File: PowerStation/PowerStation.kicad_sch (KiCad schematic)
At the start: 0 parts

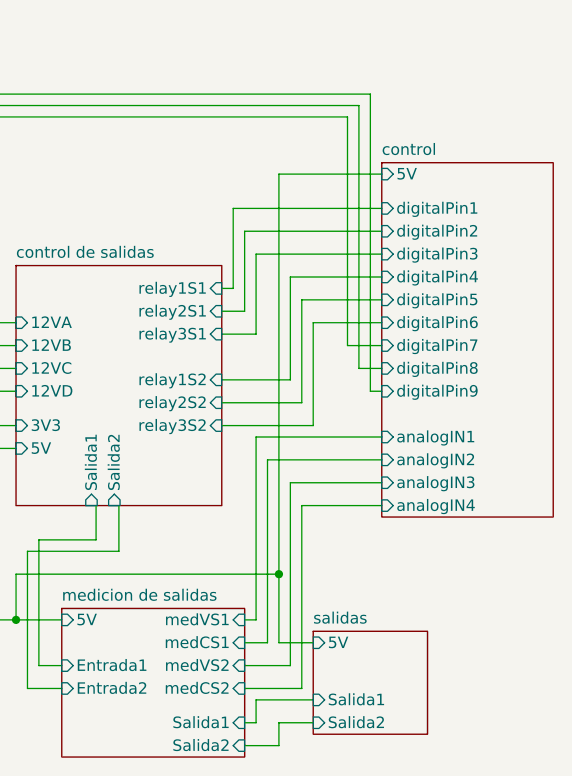
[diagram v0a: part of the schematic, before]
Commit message: correccion de esquermatico y avanze en placa
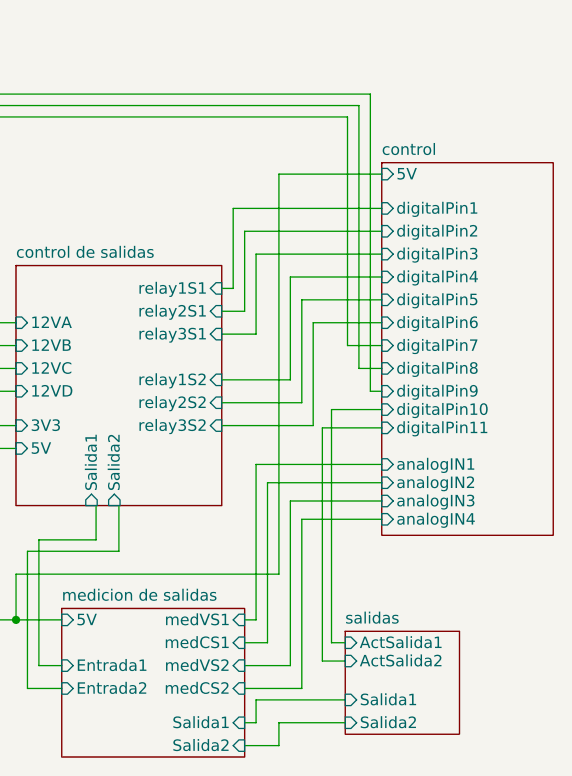
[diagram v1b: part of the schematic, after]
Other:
- sheet control ports: added digitalPin10, digitalPin11; removed none
- sheet salidas ports: added ActSalida1, ActSalida2; removed 5V
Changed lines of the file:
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@@
 (kicad_sch (version 20230121) (generator eeschema)
   (paper "A4")
-  (junction (at 161.29 111.76) (diameter 0) (color 0 0 0 0)
-  )
   (junction (at 132.08 116.84) (diameter 0) (color 0 0 0 0)
   )
-  (wire (pts (xy 165.1 119.38) (xy 161.29 119.38))
-    (stroke (width 0) (type default))
-  )
   (wire (pts (xy 163.83 92.71) (xy 163.83 81.28))
     (stroke (width 0) (type default))
   )
-  (wire (pts (xy 158.75 96.52) (xy 172.72 96.52))
+  (wire (pts (xy 158.75 99.568) (xy 172.72 99.568))
     (stroke (width 0) (type default))
   )
@@
     (stroke (width 0) (type default))
   )
-  (wire (pts (xy 163.83 124.46) (xy 163.83 104.14))
+  (wire (pts (xy 163.83 124.46) (xy 163.83 105.664))
     (stroke (width 0) (type default))
   )
@@
     (stroke (width 0) (type default))
   )
+  (wire (pts (xy 167.132 93.472) (xy 167.132 119.38))
+    (stroke (width 0) (type default))
+  )
   (wire (pts (xy 134.62 107.95) (xy 134.62 121.92))
     (stroke (width 0) (type default))
@@
     (stroke (width 0) (type default))
   )
+  (wire (pts (xy 166.116 121.412) (xy 168.656 121.412))
+    (stroke (width 0) (type default))
+  )
   (wire (pts (xy 129.54 97.79) (xy 129.54 111.76))
     (stroke (width 0) (type default))
@@
     (stroke (width 0) (type default))
   )
-  (wire (pts (xy 160.02 99.06) (xy 172.72 99.06))
+  (wire (pts (xy 160.02 101.6) (xy 172.72 101.6))
     (stroke (width 0) (type default))
   )
@@
     (stroke (width 0) (type default))
   )
+  (wire (pts (xy 172.72 93.472) (xy 167.132 93.472))
+    (stroke (width 0) (type default))
+  )
   (wire (pts (xy 162.56 90.17) (xy 162.56 78.74))
     (stroke (width 0) (type default))
@@
     (stroke (width 0) (type default))
   )
+  (wire (pts (xy 166.116 95.504) (xy 166.116 121.412))
+    (stroke (width 0) (type default))
+  )
   (wire (pts (xy 157.48 73.66) (xy 172.72 73.66))
     (stroke (width 0) (type default))
@@
     (stroke (width 0) (type default))
   )
-  (wire (pts (xy 163.83 104.14) (xy 172.72 104.14))
-    (stroke (width 0) (type default))
-  )
-  (wire (pts (xy 161.29 128.27) (xy 165.1 128.27))
+  (wire (pts (xy 163.83 105.664) (xy 172.72 105.664))
+    (stroke (width 0) (type default))
+  )
+  (wire (pts (xy 161.29 128.27) (xy 168.656 128.27))
     (stroke (width 0) (type default))
   )
@@
     (stroke (width 0) (type default))
   )
+  (wire (pts (xy 167.132 119.38) (xy 168.656 119.38))
+    (stroke (width 0) (type default))
+  )
   (wire (pts (xy 157.48 128.27) (xy 158.75 128.27))
     (stroke (width 0) (type default))
@@
     (stroke (width 0) (type default))
   )
-  (wire (pts (xy 160.02 119.38) (xy 160.02 99.06))
+  (wire (pts (xy 160.02 119.38) (xy 160.02 101.6))
     (stroke (width 0) (type default))
   )
@@
     (stroke (width 0) (type default))
   )
-  (wire (pts (xy 162.56 101.6) (xy 172.72 101.6))
+  (wire (pts (xy 162.56 103.632) (xy 172.72 103.632))
     (stroke (width 0) (type default))
   )
@@
     (stroke (width 0) (type default))
   )
-  (wire (pts (xy 161.29 119.38) (xy 161.29 111.76))
-    (stroke (width 0) (type default))
-  )
   (wire (pts (xy 154.94 82.55) (xy 157.48 82.55))
     (stroke (width 0) (type default))
@@
     (stroke (width 0) (type default))
   )
+  (wire (pts (xy 172.72 95.504) (xy 166.116 95.504))
+    (stroke (width 0) (type default))
+  )
   (wire (pts (xy 156.21 80.01) (xy 156.21 71.12))
     (stroke (width 0) (type default))
@@
     (stroke (width 0) (type default))
   )
-  (wire (pts (xy 158.75 116.84) (xy 158.75 96.52))
-    (stroke (width 0) (type default))
-  )
-  (wire (pts (xy 158.75 125.73) (xy 165.1 125.73))
+  (wire (pts (xy 158.75 116.84) (xy 158.75 99.568))
+    (stroke (width 0) (type default))
+  )
+  (wire (pts (xy 158.75 125.73) (xy 168.656 125.73))
     (stroke (width 0) (type default))
   )
@@
     (stroke (width 0) (type default))
   )
-  (wire (pts (xy 162.56 121.92) (xy 162.56 101.6))
+  (wire (pts (xy 162.56 121.92) (xy 162.56 103.632))
     (stroke (width 0) (type default))
   )
@@
     )
   )
-  (sheet (at 165.1 118.11) (size 12.7 11.43) (fields_autoplaced)
+  (sheet (at 168.656 118.11) (size 12.7 11.43) (fields_autoplaced)
     (stroke (width 0.1524) (type solid))
     (fill (color 0 0 0 0.0000))
-    (property "Sheetname" "salidas" (at 165.1 117.3984 0)
+    (property "Sheetname" "salidas" (at 168.656 117.3984 0)
       (effects (font (size 1.27 1.27)) (justify left bottom))
     )
-    (property "Sheetfile" "salidas.kicad_sch" (at 165.1 129.6166 0)
+    (property "Sheetfile" "salidas.kicad_sch" (at 168.656 129.6166 0)
       (effects (font (size 1.27 1.27)) (justify left top) hide)
     )
-    (pin "5V" input (at 165.1 119.38 180)
-      (effects (font (size 1.27 1.27)) (justify left))
-    )
-    (pin "Salida1" input (at 165.1 125.73 180)
-      (effects (font (size 1.27 1.27)) (justify left))
-    )
-    (pin "Salida2" input (at 165.1 128.27 180)
+    (pin "Salida1" input (at 168.656 125.73 180)
+      (effects (font (size 1.27 1.27)) (justify left))
+    )
+    (pin "Salida2" input (at 168.656 128.27 180)
+      (effects (font (size 1.27 1.27)) (justify left))
+    )
+    (pin "ActSalida2" input (at 168.656 121.412 180)
+      (effects (font (size 1.27 1.27)) (justify left))
+    )
+    (pin "ActSalida1" input (at 168.656 119.38 180)
       (effects (font (size 1.27 1.27)) (justify left))
     )
@@
     )
   )
-  (sheet (at 172.72 66.04) (size 19.05 39.37) (fields_autoplaced)
+  (sheet (at 172.72 66.04) (size 19.05 41.402) (fields_autoplaced)
     (stroke (width 0.1524) (type solid))
     (fill (color 0 0 0 0.0000))
@@
       (effects (font (size 1.27 1.27)) (justify left bottom))
     )
-    (property "Sheetfile" "control.kicad_sch" (at 172.72 106.2486 0)
+    (property "Sheetfile" "control.kicad_sch" (at 172.72 108.0266 0)
       (effects (font (size 1.27 1.27)) (justify left top) hide)
     )
@@
       (effects (font (size 1.27 1.27)) (justify left))
     )
-    (pin "analogIN2" input (at 172.72 99.06 180)
-      (effects (font (size 1.27 1.27)) (justify left))
-    )
-    (pin "analogIN1" input (at 172.72 96.52 180)
-      (effects (font (size 1.27 1.27)) (justify left))
-    )
-    (pin "analogIN3" input (at 172.72 101.6 180)
-      (effects (font (size 1.27 1.27)) (justify left))
-    )
-    (pin "analogIN4" input (at 172.72 104.14 180)
+    (pin "analogIN2" input (at 172.72 101.6 180)
+      (effects (font (size 1.27 1.27)) (justify left))
+    )
+    (pin "analogIN1" input (at 172.72 99.568 180)
+      (effects (font (size 1.27 1.27)) (justify left))
+    )
+    (pin "analogIN3" input (at 172.72 103.632 180)
+      (effects (font (size 1.27 1.27)) (justify left))
+    )
+    (pin "analogIN4" input (at 172.72 105.664 180)
       (effects (font (size 1.27 1.27)) (justify left))
     )
@@
       (effects (font (size 1.27 1.27)) (justify left))
     )
+    (pin "digitalPin10" input (at 172.72 93.472 180)
+      (effects (font (size 1.27 1.27)) (justify left))
+    )
+    (pin "digitalPin11" input (at 172.72 95.504 180)
+      (effects (font (size 1.27 1.27)) (justify left))
+    )
